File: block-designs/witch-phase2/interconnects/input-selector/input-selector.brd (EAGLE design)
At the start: 99.1 x 66.7 mm, 43 parts, among them IC1 74LVC1G17DBV, IC10 74LVC1G17DBV, IC11 74LVC1G17DBV, IC12 74LVC1G17DBV, IC13 74LVC1G17DBV, IC14 74LVC1G17DBV, IC2 74LVC1G17DBV, IC3 74LVC1G17DBV, IC4 74LVC1G17DBV, IC5 74LVC1G17DBV, IC6 74LVC1G17DBV, IC7 74LVC1G17DBV, IC8 74LVC1G17DBV, IC9 74LVC1G17DBV

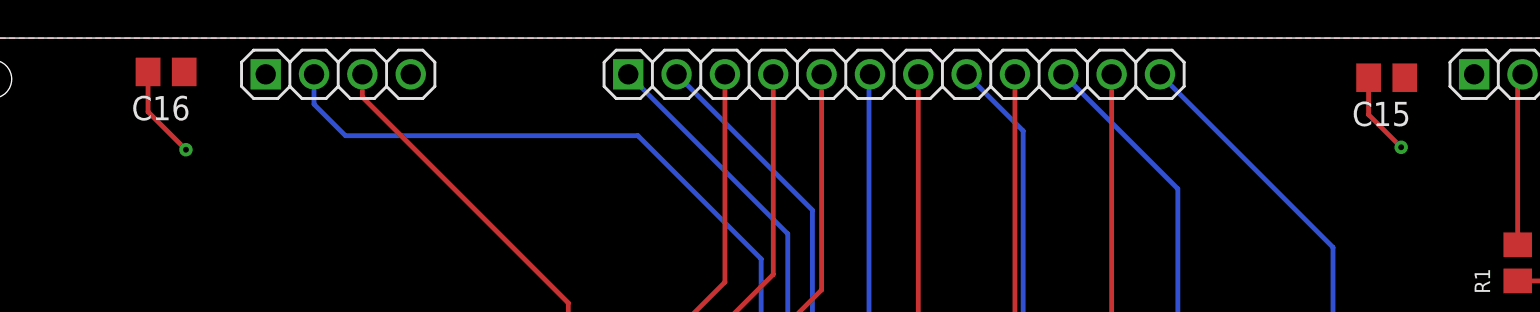
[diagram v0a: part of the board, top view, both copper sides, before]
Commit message: add revision numbers
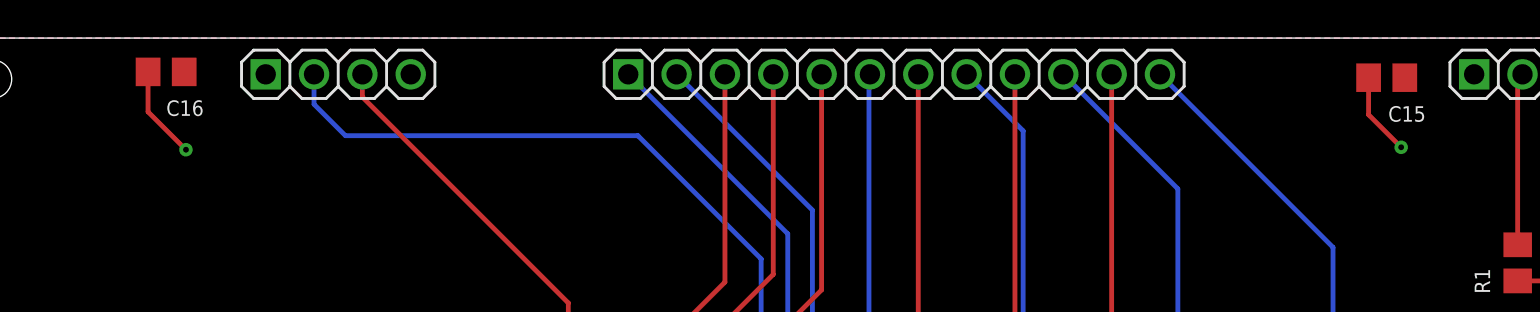
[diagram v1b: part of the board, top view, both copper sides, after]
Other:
- board text added: "Revision 1"
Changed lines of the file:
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@@
 <text x="64.008" y="5.588" size="1.778" layer="48" align="center">SND ROW</text>
 <text x="23.368" y="5.588" size="1.778" layer="48" align="center">RCV ROW</text>
-<text x="2.3876" y="56.1086" size="1.778" layer="48">Input Selector Interconnect</text>
+<text x="1.7018" y="51.7144" size="1.778" layer="48">Input Selector
+Interconnect</text>
+<text x="1.7272" y="50.0126" size="0.8128" layer="48">Revision 1</text>
 </plain>
 <attributes>
@@
 <attribute name="VALUE" x="15.748" y="-0.635" size="1.27" layer="27"/>
 </element>
-<element name="C15" library="resistor" package="C0805" value="" x="75.4126" y="64.5922" rot="R180"/>
-<element name="C16" library="resistor" package="C0805" value="" x="11.2776" y="64.897" rot="R180"/>
+<element name="C15" library="resistor" package="C0805" value="" x="75.4126" y="64.5922" smashed="yes" rot="R180">
+<attribute name="NAME" x="77.47" y="63.0936" size="0.8128" layer="25" rot="R180"/>
+<attribute name="VALUE" x="76.6826" y="67.1322" size="1.27" layer="27" rot="R180"/>
+</element>
+<element name="C16" library="resistor" package="C0805" value="" x="11.2776" y="64.897" smashed="yes" rot="R180">
+<attribute name="NAME" x="13.2588" y="63.3984" size="0.8128" layer="25" rot="R180"/>
+<attribute name="VALUE" x="12.5476" y="67.437" size="1.27" layer="27" rot="R180"/>
+</element>
 <element name="C17" library="resistor" package="C0603" value="" x="13.6652" y="3.3909" smashed="yes" rot="R270">
 <attribute name="NAME" x="12.7889" y="5.207" size="0.8128" layer="25"/>
